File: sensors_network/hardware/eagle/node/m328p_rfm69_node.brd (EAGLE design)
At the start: 64 x 38.9 mm, 32 parts, among them IC2 L6920TSSOP8, U1 ATMEGA328P_TQFP, U2 RFM69W, Y1 8MHz

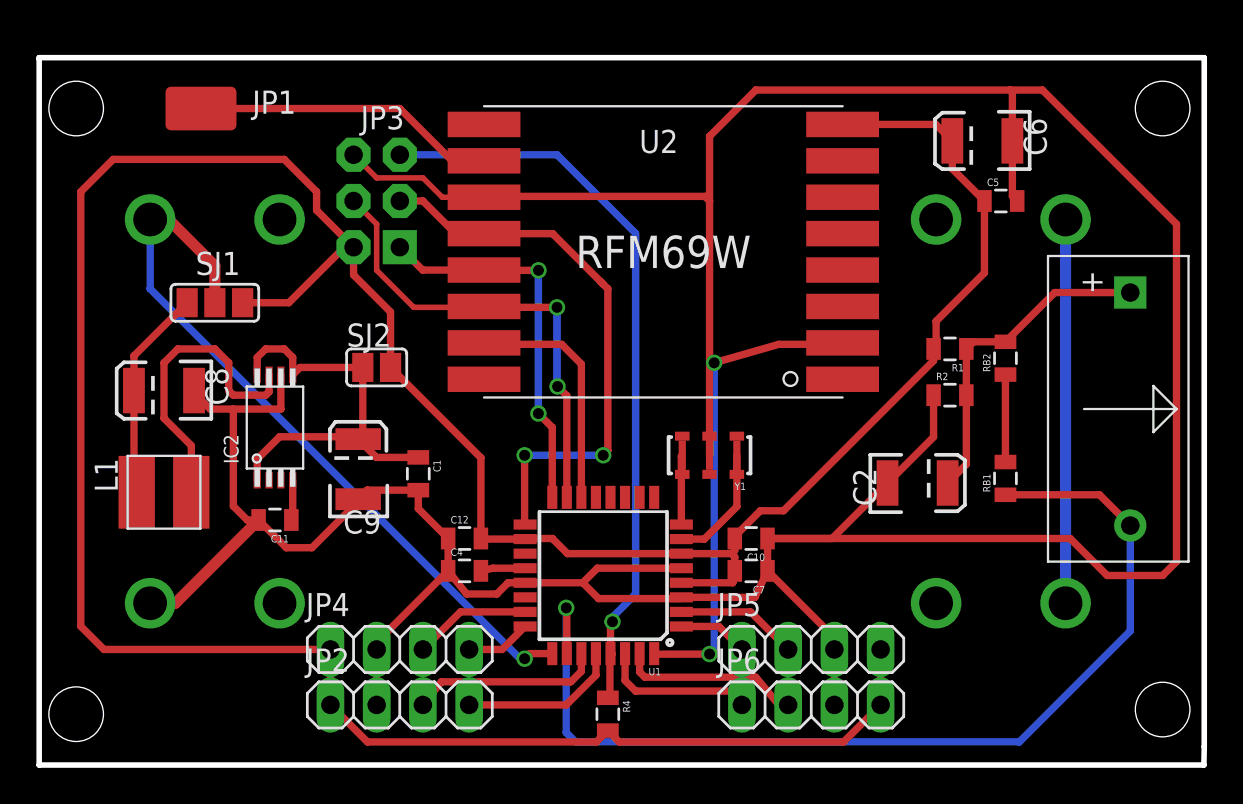
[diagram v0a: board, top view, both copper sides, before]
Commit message: [sensors network] Worked sensor node eagle design - 4th stage
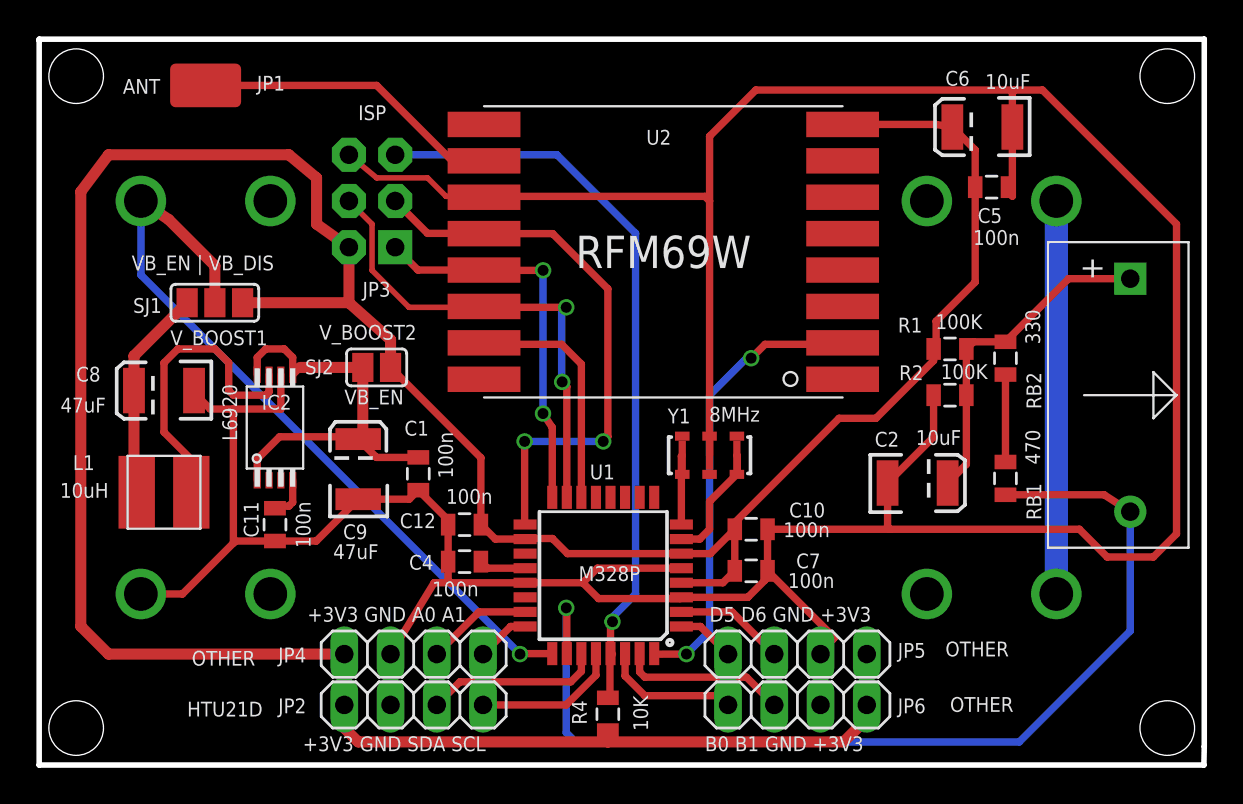
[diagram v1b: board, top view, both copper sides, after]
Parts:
- IC2: value L6920TSSOP8 -> L6920
- JP3: value AVR_SPI_PRG_6NS -> ISP
- U1: value ATMEGA328P_TQFP -> M328P
- moved JP1 1.30 mm to (8.13, 36.3)
- moved BAT3 1.14 mm to (29.7, 30.0)
- moved C5 0.92 mm to (51.3, 30.7)
- moved JP4 0.80 mm to (19.6, 5.08)
- moved JP5 0.80 mm to (40.6, 5.08)
- moved C12 0.76 mm to (22.4, 12.2)
- moved C6 0.76 mm to (50.8, 34.0)
- moved JP2 0.76 mm to (19.6, 2.29)
- moved JP6 0.76 mm to (40.6, 2.29)
- moved CT1 0.76 mm to (58.9, 19.3)
- moved BAT4 0.72 mm to (29.7, 8.38)
- moved C10 0.51 mm to (38.1, 11.9)
- moved C4 0.51 mm to (22.4, 10.2)
- moved JP3 0.25 mm to (17.3, 30.0)
- moved C11 0.25 mm to (11.9, 12.2), turned to 270 degrees
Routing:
- net GND: track 213.9 -> 205.7 mm
- net BATT_LVL: track 40.8 -> 42.8 mm
- net INT: track 26.4 -> 25.1 mm
- net MOSI: track 25.8 -> 27.0 mm
- net B0: track 8.55 -> 7.54 mm
- net SDA: track 10.5 -> 9.68 mm
- net B1: track 10.0 -> 9.16 mm
- net SCL: track 8.83 -> 8.07 mm
- net D5: track 3.85 -> 3.19 mm
- net A0: track 6.47 -> 5.81 mm
- net D6: track 6.72 -> 6.07 mm
- net A1: track 3.60 -> 2.94 mm
- net +3V3: track 176.2 -> 176.7 mm
- net N$8: track 21.1 -> 21.6 mm
- removed copper zone on layer 16, net GND
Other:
- board size 64 x 38.9 mm -> 64 x 39.9 mm
- board text added: "+3V3 GND A0 A1"
- board text added: "+3V3 GND SDA SCL"
- board text added: "B0 B1 GND +3V3"
- board text added: "D5 D6 GND +3V3"
- board text added: "VB_EN"
- board text added: "VB_EN | VB_DIS"
